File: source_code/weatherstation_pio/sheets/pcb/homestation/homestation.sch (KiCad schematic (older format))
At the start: 1 part

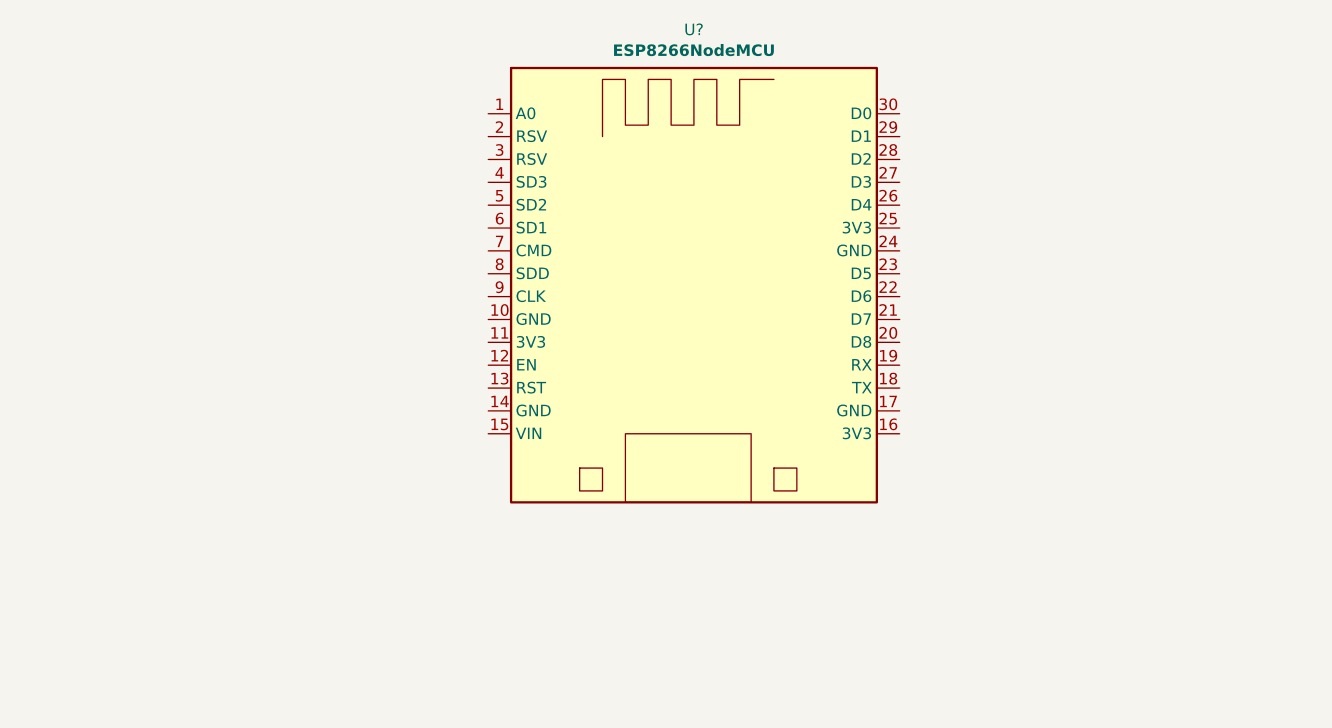
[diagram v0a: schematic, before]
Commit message: Home station finalized and report finalized.
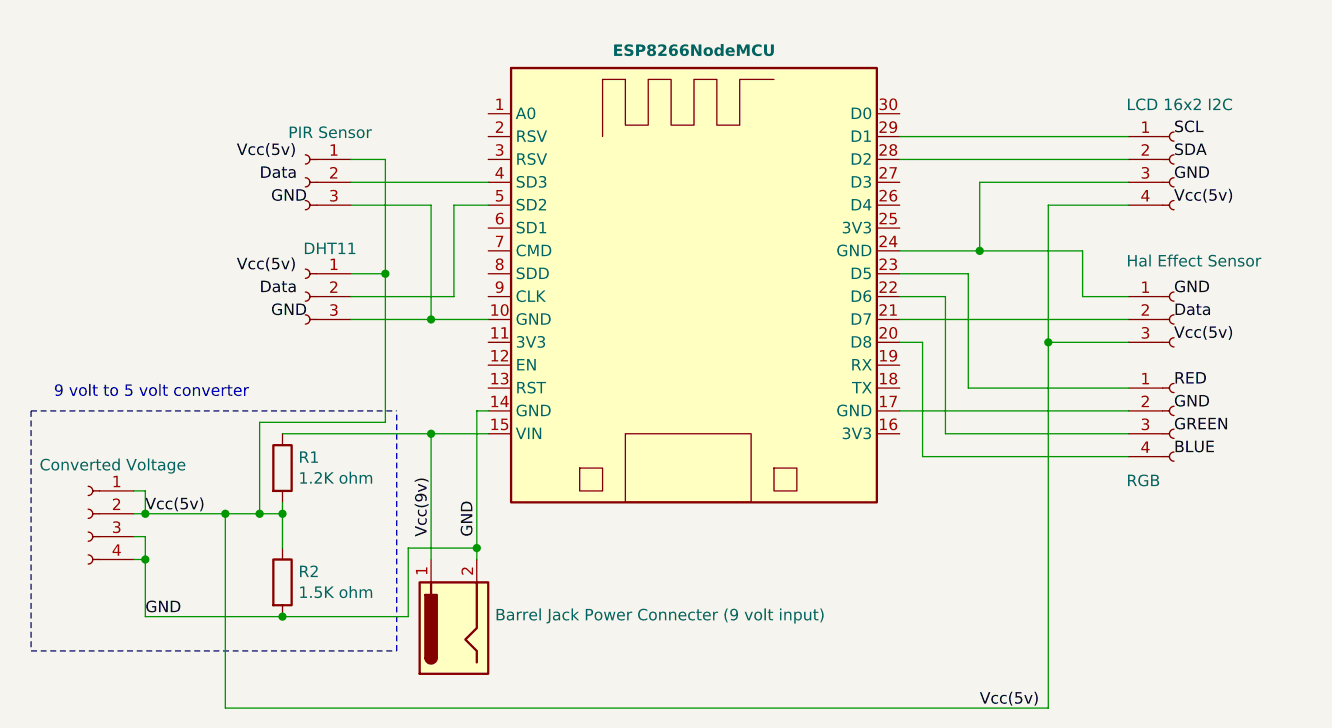
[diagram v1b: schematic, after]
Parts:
- added J1: Converted Voltage, Connector_PinHeader_2.54mm:PinHeader_1x04_P2.54mm_Vertical, symbol Connector:Conn_01x04_Female
- added J2: PIR Sensor, Connector_PinHeader_2.54mm:PinHeader_1x03_P2.54mm_Vertical, symbol Connector:Conn_01x03_Female
- added J3: DHT11, Connector_PinHeader_2.54mm:PinHeader_1x03_P2.54mm_Vertical, symbol Connector:Conn_01x03_Female
- added J4: Barrel Jack Power Connecter (9 volt input), Connector_BarrelJack:BarrelJack_Horizontal, symbol Connector:Barrel_Jack
- added J5: LCD 16x2 I2C, Connector_PinHeader_2.54mm:PinHeader_1x04_P2.54mm_Vertical, symbol Connector:Conn_01x04_Female
- added J6: Hal Effect Sensor, Connector_PinHeader_2.54mm:PinHeader_1x03_P2.54mm_Vertical, symbol Connector:Conn_01x03_Female
- added J7: RGB, Connector_PinHeader_2.54mm:PinHeader_1x04_P2.54mm_Vertical, symbol Connector:Conn_01x04_Female
- added R1: 1.2K ohm, Resistor_THT:R_Axial_DIN0204_L3.6mm_D1.6mm_P7.62mm_Horizontal, symbol Device:R
- added R2: 1.5K ohm, Resistor_THT:R_Axial_DIN0204_L3.6mm_D1.6mm_P7.62mm_Horizontal, symbol Device:R
- U1: renamed from U?; footprint smart_things_PCBv1:ESP8266_nodeMCU_V1 -> esp8266_nodemcu:ESP8266_nodeMCU_V1
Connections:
- net at U1.10 (GND): now also J2.3 (Pin_3), J3.3 (Pin_3)
- net GND: now reaches U1.14 (GND)
- net GND: now also J1.3 (Pin_3), J1.4 (Pin_4), J4.2, R2.2
- net Vcc(9v): now reaches U1.15 (VIN)
- net Vcc(9v): now also J4.1, R1.1
- net at U1.17 (GND): now also J7.2 (Pin_2)
- net at U1.20 (D8): now also J7.4 (Pin_4)
- net at U1.21 (D7): now also J6.2 (Pin_2)
- net at U1.22 (D6): now also J7.3 (Pin_3)
- net at U1.23 (D5): now also J7.1 (Pin_1)
- net at U1.24 (GND): now also J5.3 (Pin_3), J6.1 (Pin_1)
- net at U1.28 (D2): now also J5.2 (Pin_2)
- net at U1.29 (D1): now also J5.1 (Pin_1)
- net at U1.4 (SD3): now also J2.2 (Pin_2)
- net at U1.5 (SD2): now also J3.2 (Pin_2)
- new net Vcc(5v): J1.1 (Pin_1), J1.2 (Pin_2), J2.1 (Pin_1), J3.1 (Pin_1), J5.4 (Pin_4), J6.3 (Pin_3), R1.2, R2.1
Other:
- note added: "9 volt to 5 volt converter"
